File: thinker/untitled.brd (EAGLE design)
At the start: 56 x 65 mm, 2 parts

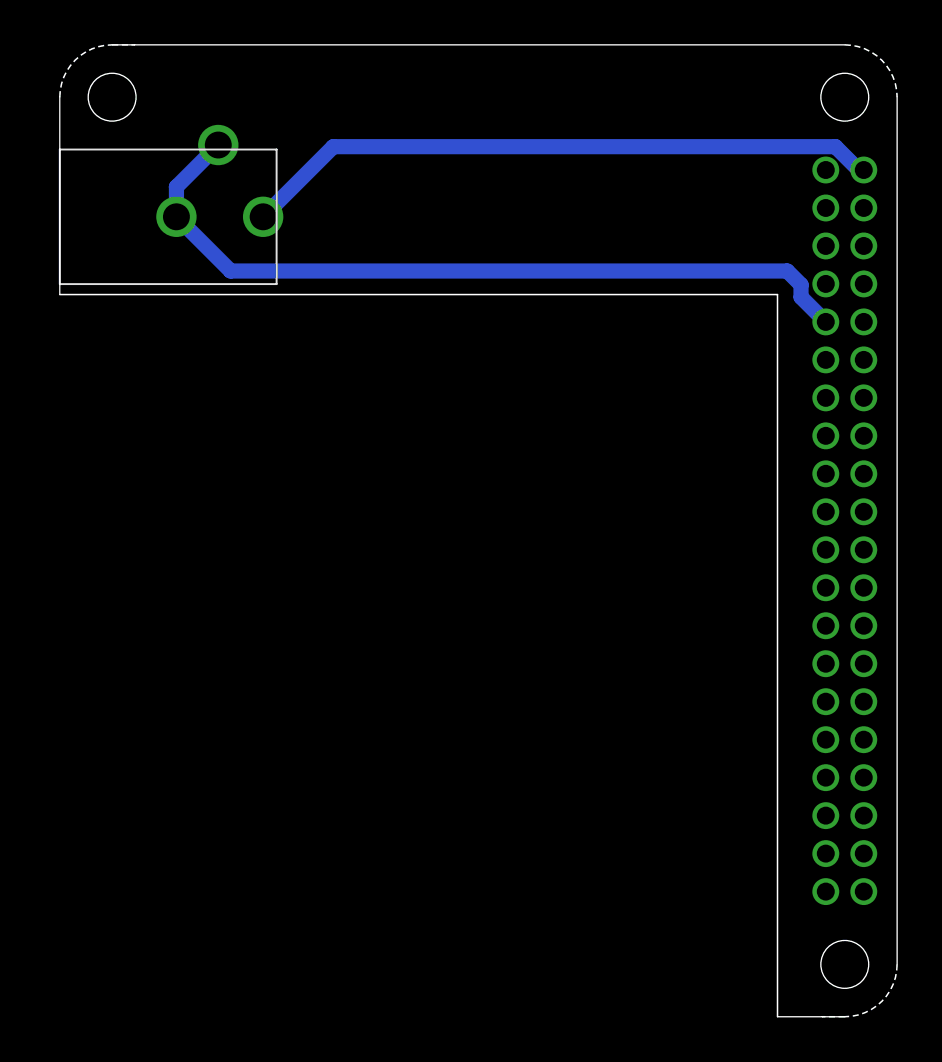
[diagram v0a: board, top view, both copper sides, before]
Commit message: Add files via upload
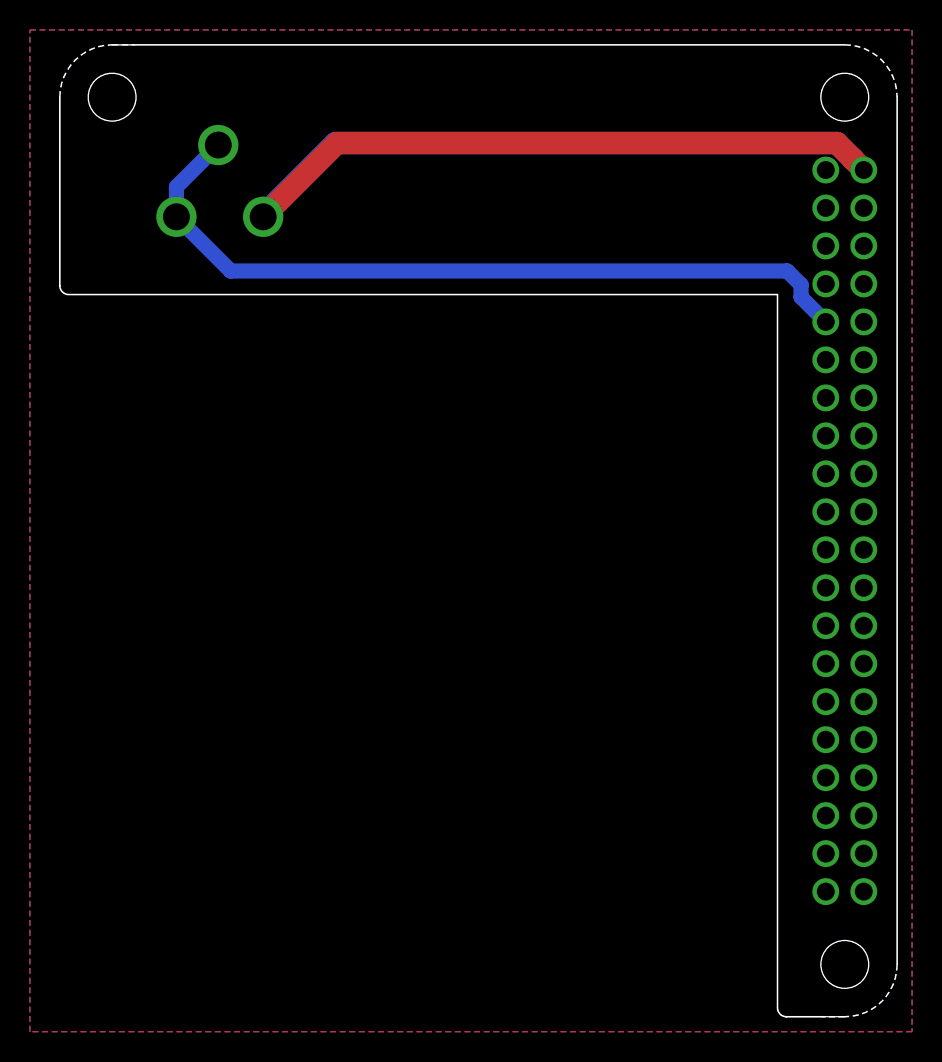
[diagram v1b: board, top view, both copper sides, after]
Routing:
- net N$1: track 42.8 -> 85.9 mm
- added copper zone on layer 1, net N$2
- added copper zone on layer 16, net N$2
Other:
- outline, holes or cut-outs redrawn
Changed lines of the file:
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@@
 <setting verticaltext="up"/>
 </settings>
-<grid distance="1" unitdist="mm" unit="mm" style="lines" multiple="1" display="no" altdistance="5" altunitdist="mil" altunit="mil"/>
+<grid distance="1" unitdist="mm" unit="mm" style="lines" multiple="1" display="no" altdistance="0.1" altunitdist="mm" altunit="mm"/>
 <layers>
 <layer number="1" name="Top" color="4" fill="1" visible="yes" active="yes"/>
@@
 <board>
 <plain>
-<wire x1="48" y1="0" x2="51" y2="0" width="0" layer="20"/>
+<wire x1="48.6" y1="0" x2="51" y2="0" width="0.106" layer="20"/>
 <wire x1="51" y1="0" x2="52.5" y2="0" width="0" layer="20"/>
-<wire x1="56" y1="3.5" x2="56" y2="61.5" width="0" layer="20"/>
-<wire x1="52.5" y1="65" x2="5" y2="65" width="0" layer="20"/>
+<wire x1="56" y1="3.5" x2="56" y2="61.5" width="0.106" layer="20"/>
+<wire x1="52.5" y1="65" x2="5" y2="65" width="0.106" layer="20"/>
 <wire x1="5" y1="65" x2="3.5" y2="65" width="0" layer="20"/>
-<wire x1="0" y1="61.5" x2="0" y2="48.3" width="0" layer="20"/>
-<wire x1="0" y1="48.3" x2="48" y2="48.3" width="0.1016" layer="20"/>
-<wire x1="48" y1="48.3" x2="48" y2="0" width="0.1016" layer="20"/>
+<wire x1="0" y1="61.5" x2="0" y2="48.9" width="0.106" layer="20"/>
+<wire x1="0.6" y1="48.3" x2="48" y2="48.3" width="0.1016" layer="20"/>
+<wire x1="48" y1="48.3" x2="48" y2="0.6" width="0.1016" layer="20"/>
 <hole x="3.5" y="61.5" drill="3.2"/>
 <hole x="52.5" y="61.5" drill="3.2"/>
@@
 <wire x1="56" y1="3.5" x2="52.5" y2="0" width="0.1016" layer="20" style="shortdash" curve="-90"/>
 <wire x1="52.5" y1="0" x2="51" y2="0" width="0.1016" layer="20" style="shortdash"/>
+<wire x1="0.6" y1="48.3" x2="0" y2="48.9" width="0.106" layer="20" curve="-90"/>
+<wire x1="48.6" y1="0" x2="48" y2="0.6" width="0.106" layer="20" curve="-90"/>
 </plain>
 <attributes>
@@
 </class>
 </classes>
-<designrules name="default">
+<designrules name="default *">
 <description language="de">&lt;b&gt;EAGLE Design Rules&lt;/b&gt;
 &lt;p&gt;
@@
 <param name="mdViaViaSameLayer" value="6mil"/>
 <param name="mnLayersViaInSmd" value="2"/>
-<param name="mdCopperDimension" value="40mil"/>
+<param name="mdCopperDimension" value="20mil"/>
 <param name="mdDrill" value="6mil"/>
 <param name="mdSmdStop" value="0mil"/>
@@
 <contactref element="U$2" pad="5V_"/>
 <contactref element="U$1" pad="VCC"/>
-<wire x1="53.43674375" y1="56.63" x2="53.77" y2="56.63" width="1.016" layer="16"/>
-<wire x1="51.87634375" y1="58.1904" x2="53.43674375" y2="56.63" width="1.016" layer="16"/>
-<wire x1="18.2904" y1="58.1904" x2="51.87634375" y2="58.1904" width="1.016" layer="16"/>
-<wire x1="13.6" y1="53.5" x2="18.2904" y2="58.1904" width="1.016" layer="16"/>
+<wire x1="13.57658125" y1="53.5676" x2="13.5676" y2="53.5676" width="1.5" layer="16"/>
+<wire x1="51.97658125" y1="58.4324" x2="53.0324" y2="57.37658125" width="1.5" layer="1" locked="yes"/>
+<wire x1="53.0324" y1="57.37658125" x2="53.0324" y2="57.3676" width="1.5" layer="1"/>
+<wire x1="53.0324" y1="57.3676" x2="53.77" y2="56.63" width="1.5" layer="1" locked="yes"/>
+<wire x1="18.5324" y1="58.4324" x2="51.97658125" y2="58.4324" width="1.5" layer="1" locked="yes"/>
+<wire x1="13.6" y1="53.5" x2="18.5324" y2="58.4324" width="1.5" layer="1" locked="yes"/>
+<wire x1="53.0324" y1="57.37658125" x2="51.97658125" y2="58.4324" width="1.5" layer="16"/>
+<wire x1="53.77" y1="56.63" x2="53.0324" y2="57.3676" width="1.5" layer="16"/>
+<wire x1="53.0324" y1="57.3676" x2="53.0324" y2="57.37658125" width="1.5" layer="16"/>
+<wire x1="51.97658125" y1="58.4324" x2="18.44138125" y2="58.4324" width="1.5" layer="16"/>
+<wire x1="18.44138125" y1="58.4324" x2="13.57658125" y2="53.5676" width="1.5" layer="16"/>
 <wire x1="53.77" y1="56.63" x2="53.77" y2="54.09" width="0" layer="19" extent="1-1"/>
 </signal>
@@
 <wire x1="49.5748" y1="48.95230625" x2="49.5748" y2="48.1252" width="1.016" layer="16"/>
 <wire x1="49.5748" y1="48.1252" x2="51.23" y2="46.47" width="1.016" layer="16"/>
-<wire x1="49.5748" y1="48.95230625" x2="53.77" y2="51.55" width="0" layer="19" extent="16-16"/>
-<wire x1="53.77" y1="41.39" x2="51.23" y2="46.47" width="0" layer="19" extent="1-1"/>
-<wire x1="53.77" y1="33.77" x2="53.77" y2="41.39" width="0" layer="19" extent="1-1"/>
-<wire x1="51.23" y1="26.15" x2="53.77" y2="33.77" width="0" layer="19" extent="1-1"/>
-<wire x1="53.77" y1="21.07" x2="51.23" y2="26.15" width="0" layer="19" extent="1-1"/>
-<wire x1="53.77" y1="15.99" x2="53.77" y2="21.07" width="0" layer="19" extent="1-1"/>
-<wire x1="51.23" y1="8.37" x2="53.77" y2="15.99" width="0" layer="19" extent="1-1"/>
+<polygon width="0.1" layer="1">
+<vertex x="-2" y="66"/>
+<vertex x="57" y="66"/>
+<vertex x="57" y="-1"/>
+<vertex x="-2" y="-1"/>
+</polygon>
+<polygon width="0.1" layer="16">
+<vertex x="-2" y="66"/>
+<vertex x="57" y="66"/>
+<vertex x="57" y="-1"/>
+<vertex x="-2" y="-1"/>
+</polygon>
 </signal>
 </signals>
@@
 </board>
 </drawing>
+<compatibility>
+<note version="8.5" severity="warning">
+Since Version 8.5, EAGLE supports locking for holes, vias, wires and polygons.
+The locking property on all objects of these types will not be understood in this version.
+</note>
+</compatibility>
 </eagle>
